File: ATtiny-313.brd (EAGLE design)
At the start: 24.4 x 59.7 mm, 17 parts, among them IC1 REG1117, IC2 ATtiny85

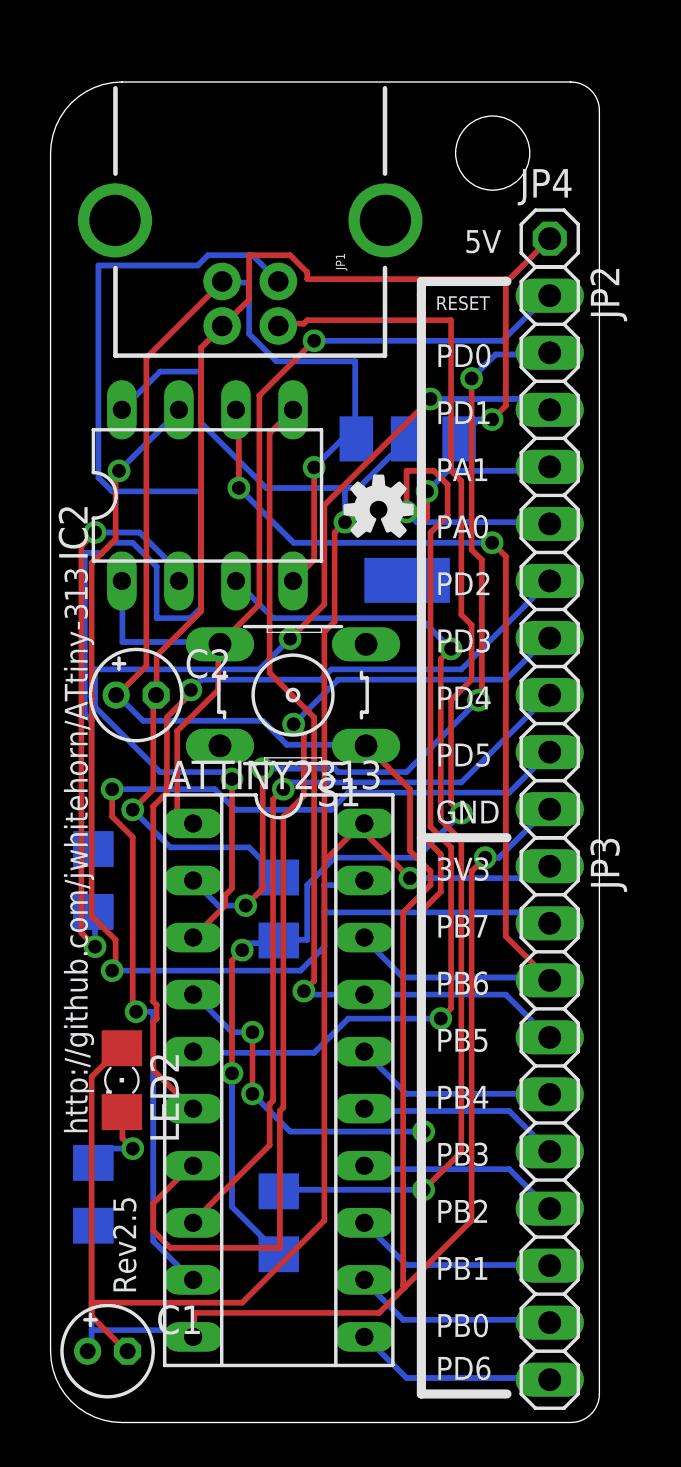
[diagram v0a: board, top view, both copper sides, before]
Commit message: work on rev 3
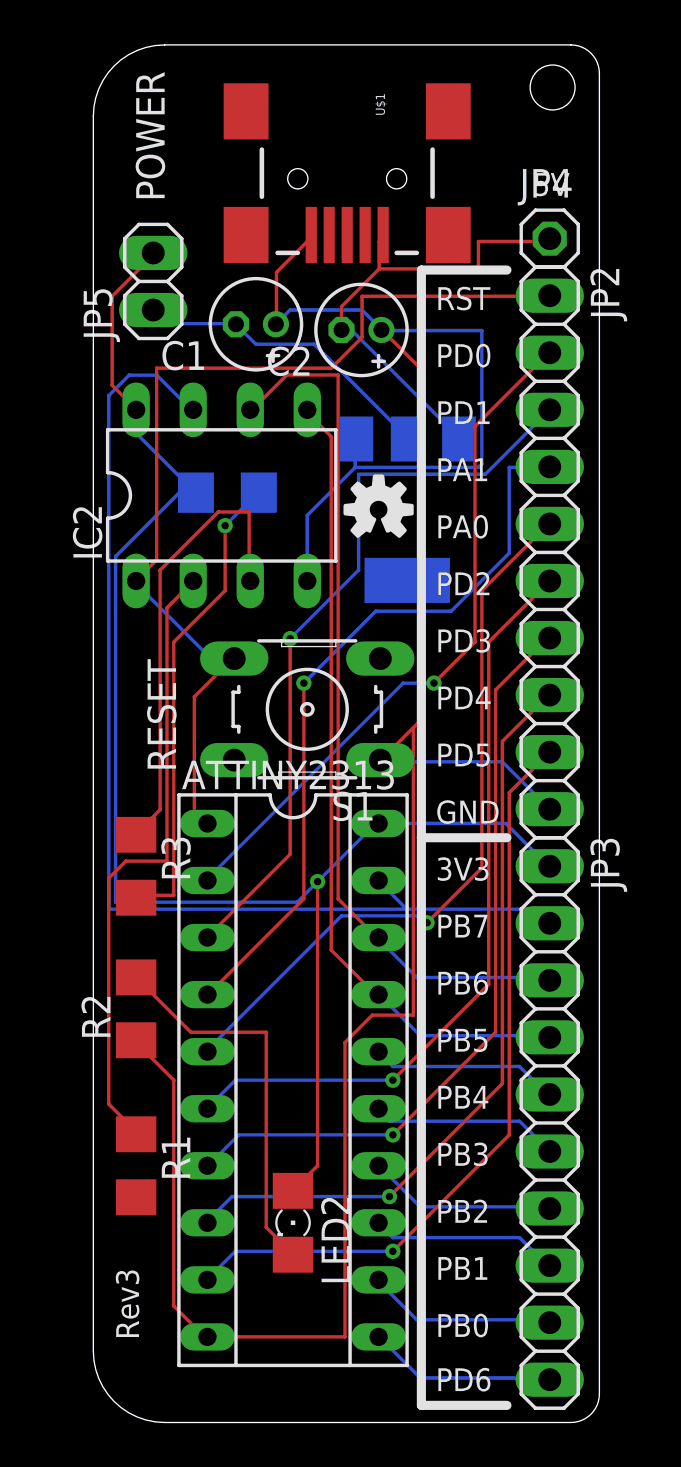
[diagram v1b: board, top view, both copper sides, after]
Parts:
- removed JP1: USB-B, SparkFun-Connectors:USB-B-PTH
- removed U$2: (no value), SparkFun-Electromechanical:STAND-OFF
- added JP5: (no value), pinhead:1X02
- added U$1: USB-MINIB-5PIN, SparkFun-Connectors:USB-MINIB
- moved C1 46.2 mm to (24.4, 56.5), turned to 180 degrees
- moved C2 19.1 mm to (29.1, 56.3), turned to 180 degrees
- moved R4 18.7 mm to (23.1, 49.0), turned to 0 degrees
- moved R3 17.1 mm to (19.1, 32.4), flipped to the top
- moved R1 12.8 mm to (19.1, 19.1), flipped to the top, turned to 270 degrees
- moved LED2 9.92 mm to (26.0, 16.5)
- moved R2 8.47 mm to (19.1, 26.0), flipped to the top
- moved S1 0.90 mm to (26.7, 39.4)
- moved ATTINY2313 0.64 mm to (26.0, 22.9)
- moved IC2 0.63 mm to (22.9, 48.9)
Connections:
- new net N$3: C1.-, IC1.2, JP5.1
- net 3.3V: now also JP5.2, R4.2; no longer C1.-, IC1.2
- net 5V: now also U$1.VBUS; no longer JP1.VBUS, R4.2
- net D+': no longer JP1.D+
- net D-': no longer JP1.D-
- net GND: now also U$1.GND; no longer JP1.GND
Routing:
- net D+': track 49.8 -> 0.00 mm
- net D-': track 59.0 -> 21.3 mm, vias 3 -> 1
- net 5V: track 57.7 -> 21.0 mm, vias 2 -> 0
- net N$2: track 42.7 -> 20.4 mm, vias 2 -> 0
- net 3.3V: track 89.7 -> 69.2 mm, vias 2 -> 1
- net N$8: track 49.7 -> 32.8 mm, vias 4 -> 1
- net N$9: track 46.8 -> 32.5 mm, vias 2 -> 1
- net N$3: track 0.00 -> 13.7 mm
- net N$24: track 3.83 -> 17.2 mm, vias 1 -> 0
- net N$11: track 46.6 -> 33.9 mm
- net N$7: track 44.9 -> 33.1 mm, vias 3 -> 1
- net GND: track 124.4 -> 112.8 mm, vias 2 -> 0
- net N$13: track 44.7 -> 33.9 mm, vias 2 -> 1
- net N$6: track 38.7 -> 30.6 mm, vias 4 -> 1
- net MISO': track 45.4 -> 38.8 mm, vias 2 -> 0
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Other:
- board size 24.4 x 59.7 mm -> 22.5 x 61.3 mm
- board text added: "POWER"
- board text added: "RST"
- board text added: "Rev3"
- board text removed: "Rev2.5"
- board text removed: "http://github.com/jwhitehorn/ATtiny-313"
